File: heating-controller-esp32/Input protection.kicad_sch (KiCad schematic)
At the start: 2 parts

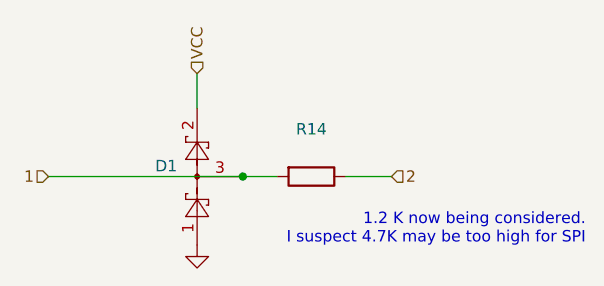
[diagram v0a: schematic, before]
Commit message: Mounting holes, a few more tweaks
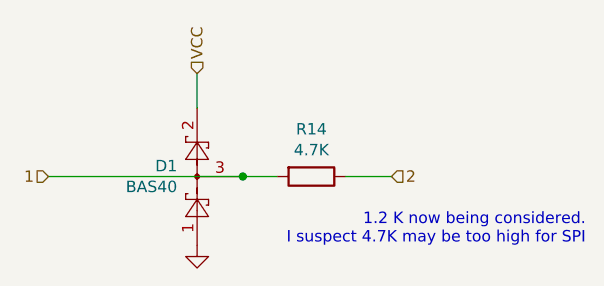
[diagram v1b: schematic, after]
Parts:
- D1: value ~ -> BAS40
- R14: value ~ -> 4.7K
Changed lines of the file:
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@@
       (effects (font (size 1.27 1.27)) (justify left))
     )
-    (property "Value" "~" (id 1) (at 86.6902 70.993 90)
+    (property "Value" "BAS40" (id 1) (at 86.6902 70.993 90)
       (effects (font (size 1.27 1.27)) (justify left))
     )
@@
     (in_bom yes) (on_board yes)
     (property "Reference" "R14" (id 0) (at 101.6 64.5922 90))
-    (property "Value" "~" (id 1) (at 101.6 66.9036 90))
+    (property "Value" "4.7K" (id 1) (at 101.6 66.9036 90))
     (property "Footprint" "Resistor_SMD:R_0603_1608Metric" (id 2) (at 101.6 68.072 90)
       (effects (font (size 1.27 1.27)) hide)
